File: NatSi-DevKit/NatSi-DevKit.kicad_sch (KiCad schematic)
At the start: 2 parts

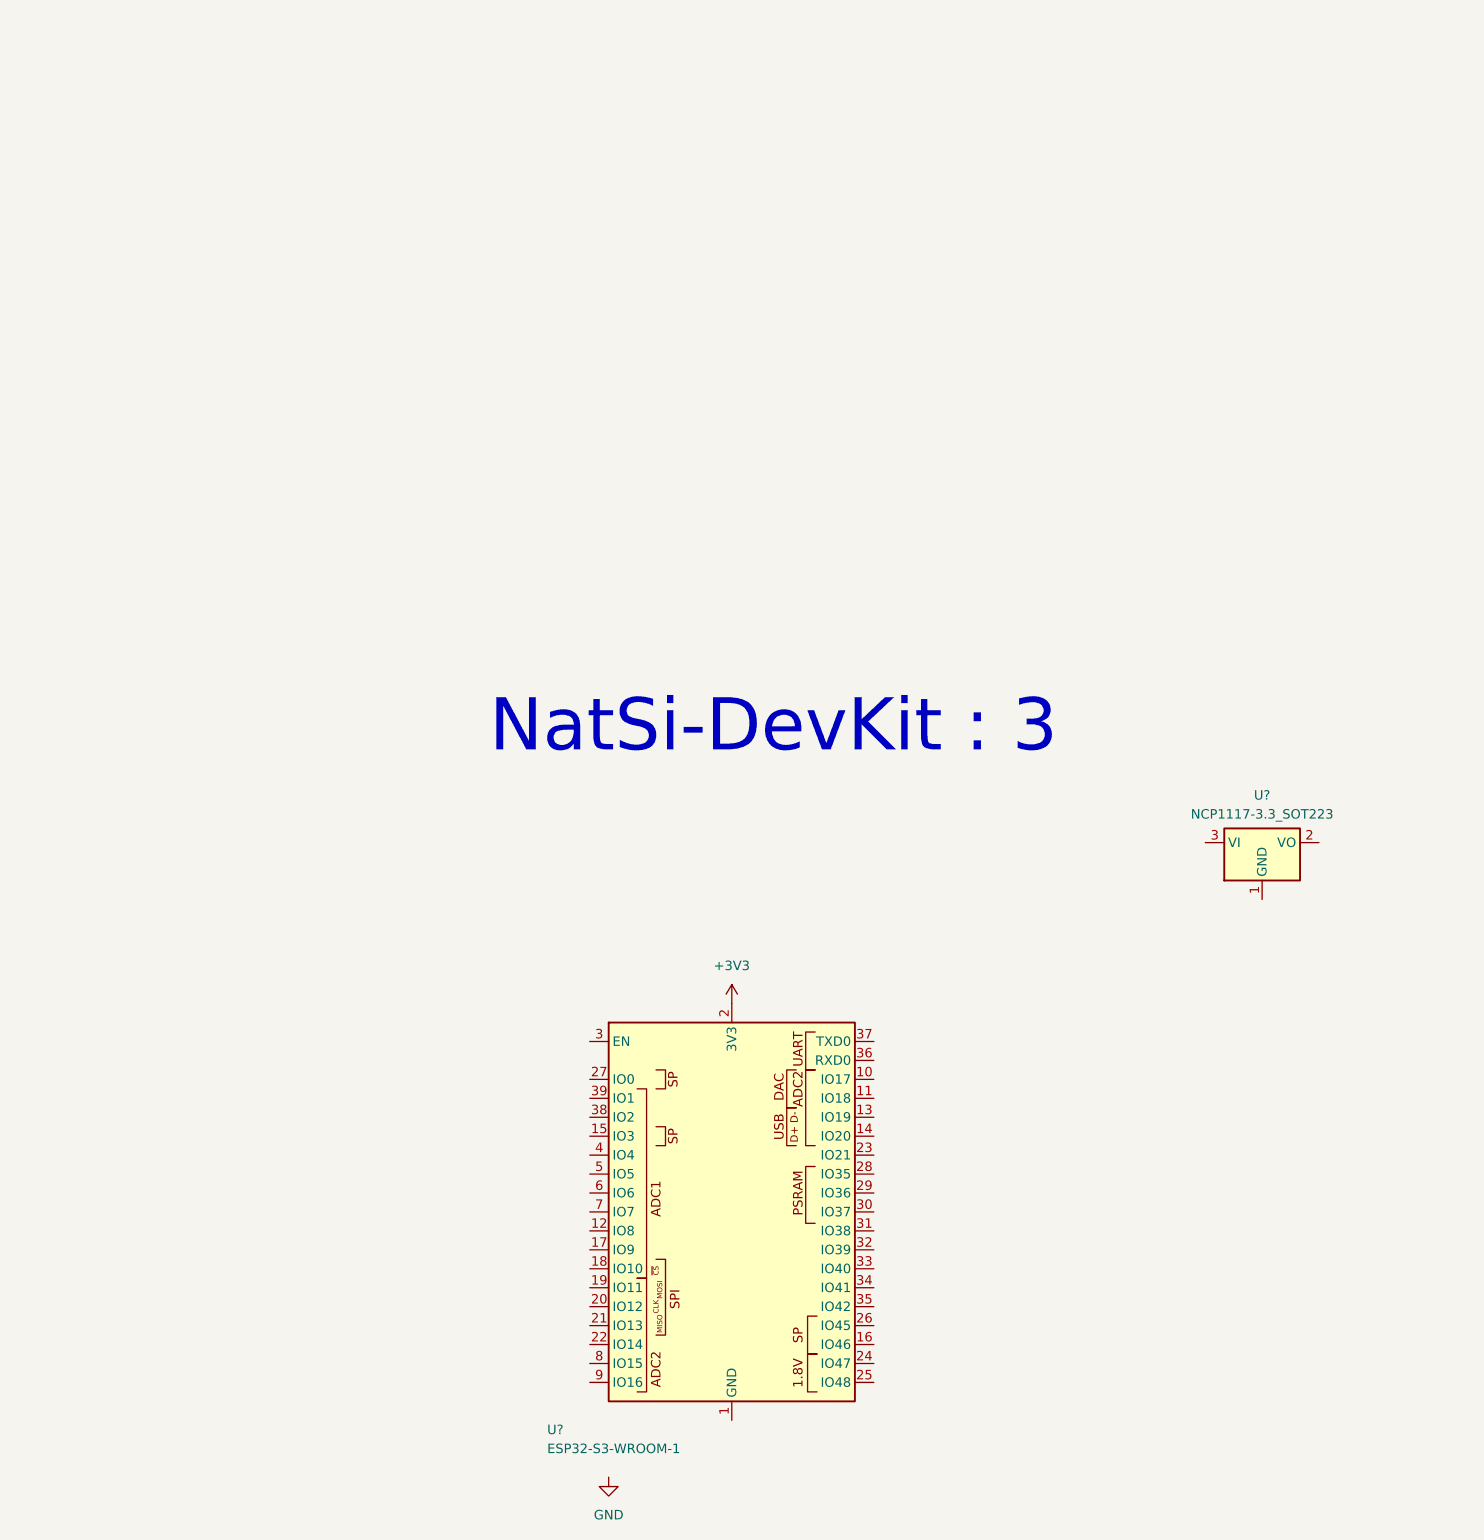
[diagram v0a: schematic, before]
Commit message: some updates schematic
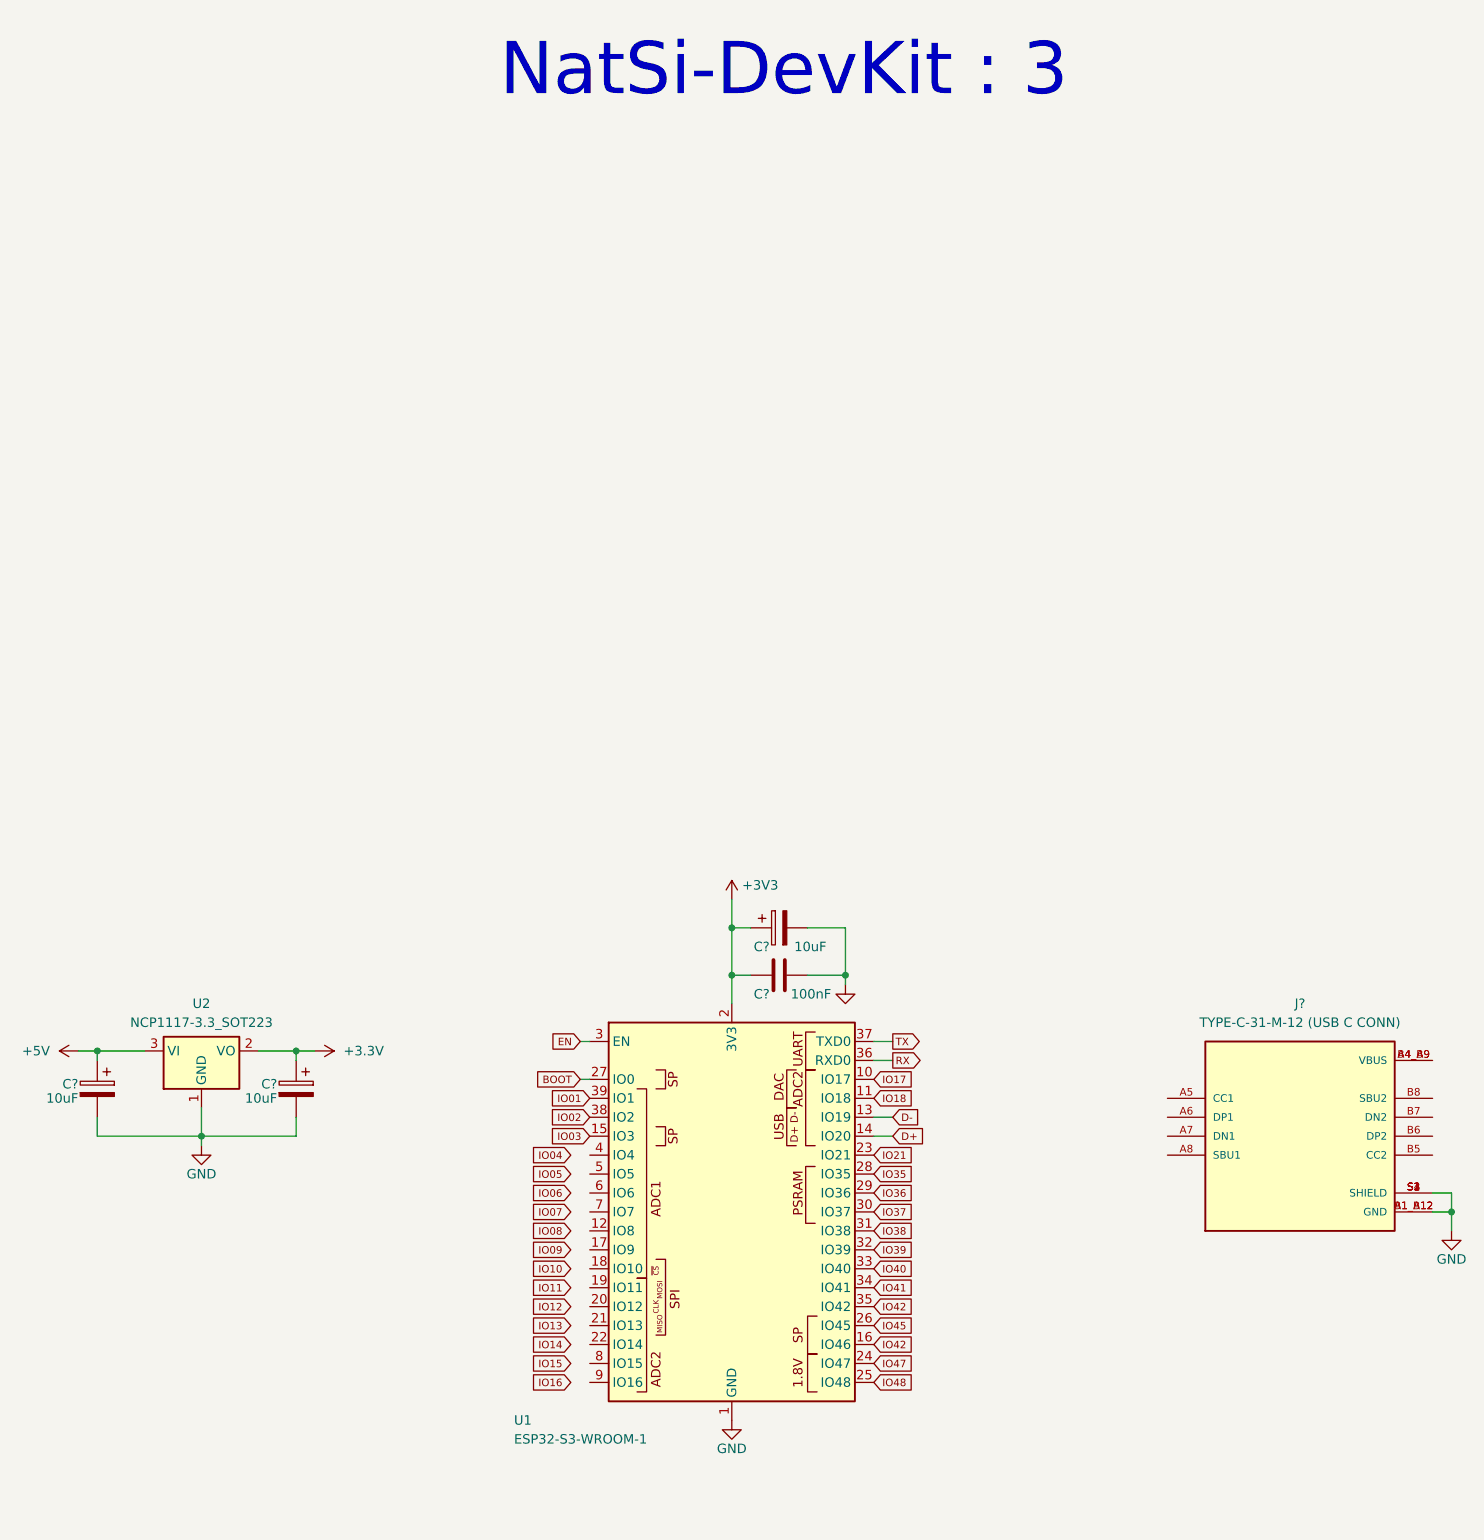
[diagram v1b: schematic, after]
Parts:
- added C? (x3): 10uF, Capacitor_Tantalum_SMD:CP_EIA-3216-18_Kemet-A_Pad1.58x1.35mm_HandSolder, symbol Device:C_Polarized
- added C?: 100nF, Capacitor_SMD:C_0805_2012Metric_Pad1.18x1.45mm_HandSolder, symbol Device:C
- added J?: TYPE-C-31-M-12 (USB C CONN), TYPE-C-31-M-12:HRO_TYPE-C-31-M-12, symbol SchrackThingy_library:TYPE-C-31-M-12 (USB C CONN)
- gave numbers to parts that had none: 2
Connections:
- net +3V3: now also C?.1, C?.1
- net GND: now also U1.1 (GND), U1.40 (GND), U1.41 (GND), U2.1 (GND), C?.2, C?.2, C?.2, C?.2, J?.A1_B12 (GND), J?.B1_A12 (GND), J?.S1 (SHIELD), J?.S2 (SHIELD), J?.S3 (SHIELD), J?.S4 (SHIELD)
- net IO17: now reaches U1.10 (IO17)
- net IO18: now reaches U1.11 (IO18)
- net D-: now reaches U1.13 (IO19)
- net D+: now reaches U1.14 (IO20)
- net IO03: now reaches U1.15 (IO3)
- net IO42: now reaches U1.16 (IO46)
- net IO42: now also U1.35 (IO42)
- net IO21: now reaches U1.23 (IO21)
- net IO47: now reaches U1.24 (IO47)
- net IO48: now reaches U1.25 (IO48)
- net IO45: now reaches U1.26 (IO45)
- net BOOT: now reaches U1.27 (IO0)
- net IO35: now reaches U1.28 (IO35)
- net IO36: now reaches U1.29 (IO36)
- net EN: now reaches U1.3 (EN)
- net IO37: now reaches U1.30 (IO37)
- net IO38: now reaches U1.31 (IO38)
- net IO39: now reaches U1.32 (IO39)
- net IO40: now reaches U1.33 (IO40)
- net IO41: now reaches U1.34 (IO41)
- net RX: now reaches U1.36 (RXD0)
- net TX: now reaches U1.37 (TXD0)
- net IO02: now reaches U1.38 (IO2)
- net IO01: now reaches U1.39 (IO1)
- net +3.3V: now reaches U2.2 (VO)
- net +3.3V: now also C?.1
- net +5V: now reaches U2.3 (VI)
- net +5V: now also C?.1
- new net: J?.A4_B9 (VBUS), J?.B4_A9 (VBUS)
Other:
- moved on the sheet: U2
